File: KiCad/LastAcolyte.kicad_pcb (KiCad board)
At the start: 2 copper layers, 170 x 170 mm, 290 parts, among them J1 USB_B, J2 Mini-DIN-6, J3 AudioJack3, J4 DB15_Female_HighDensity, J5 Conn-01x06, J6 Conn_01x02, J7 Conn_02x20_Odd_Even, Q1 PN2222A, SW1 SW_SPDT, SW2 SW_Push, U1 W65C02SxP, U10 74HC273, U11 74HC166, U12 74HC166, U13 74HC10, U14 74HC00, U15 74HC02, U16 MCP130-xxxDxTO, U17 25LCxxx, U18 W65C22SxP, U19 74HC688, U2 AS6C4008-55PCN, U20 74HC08, U3 SST39SF040, U4 74HC161, U5 74HC590, U6 74HC590, U7 74HC590, U8 74HC245, U9 74HC377, X1 CXO_DIP8/14

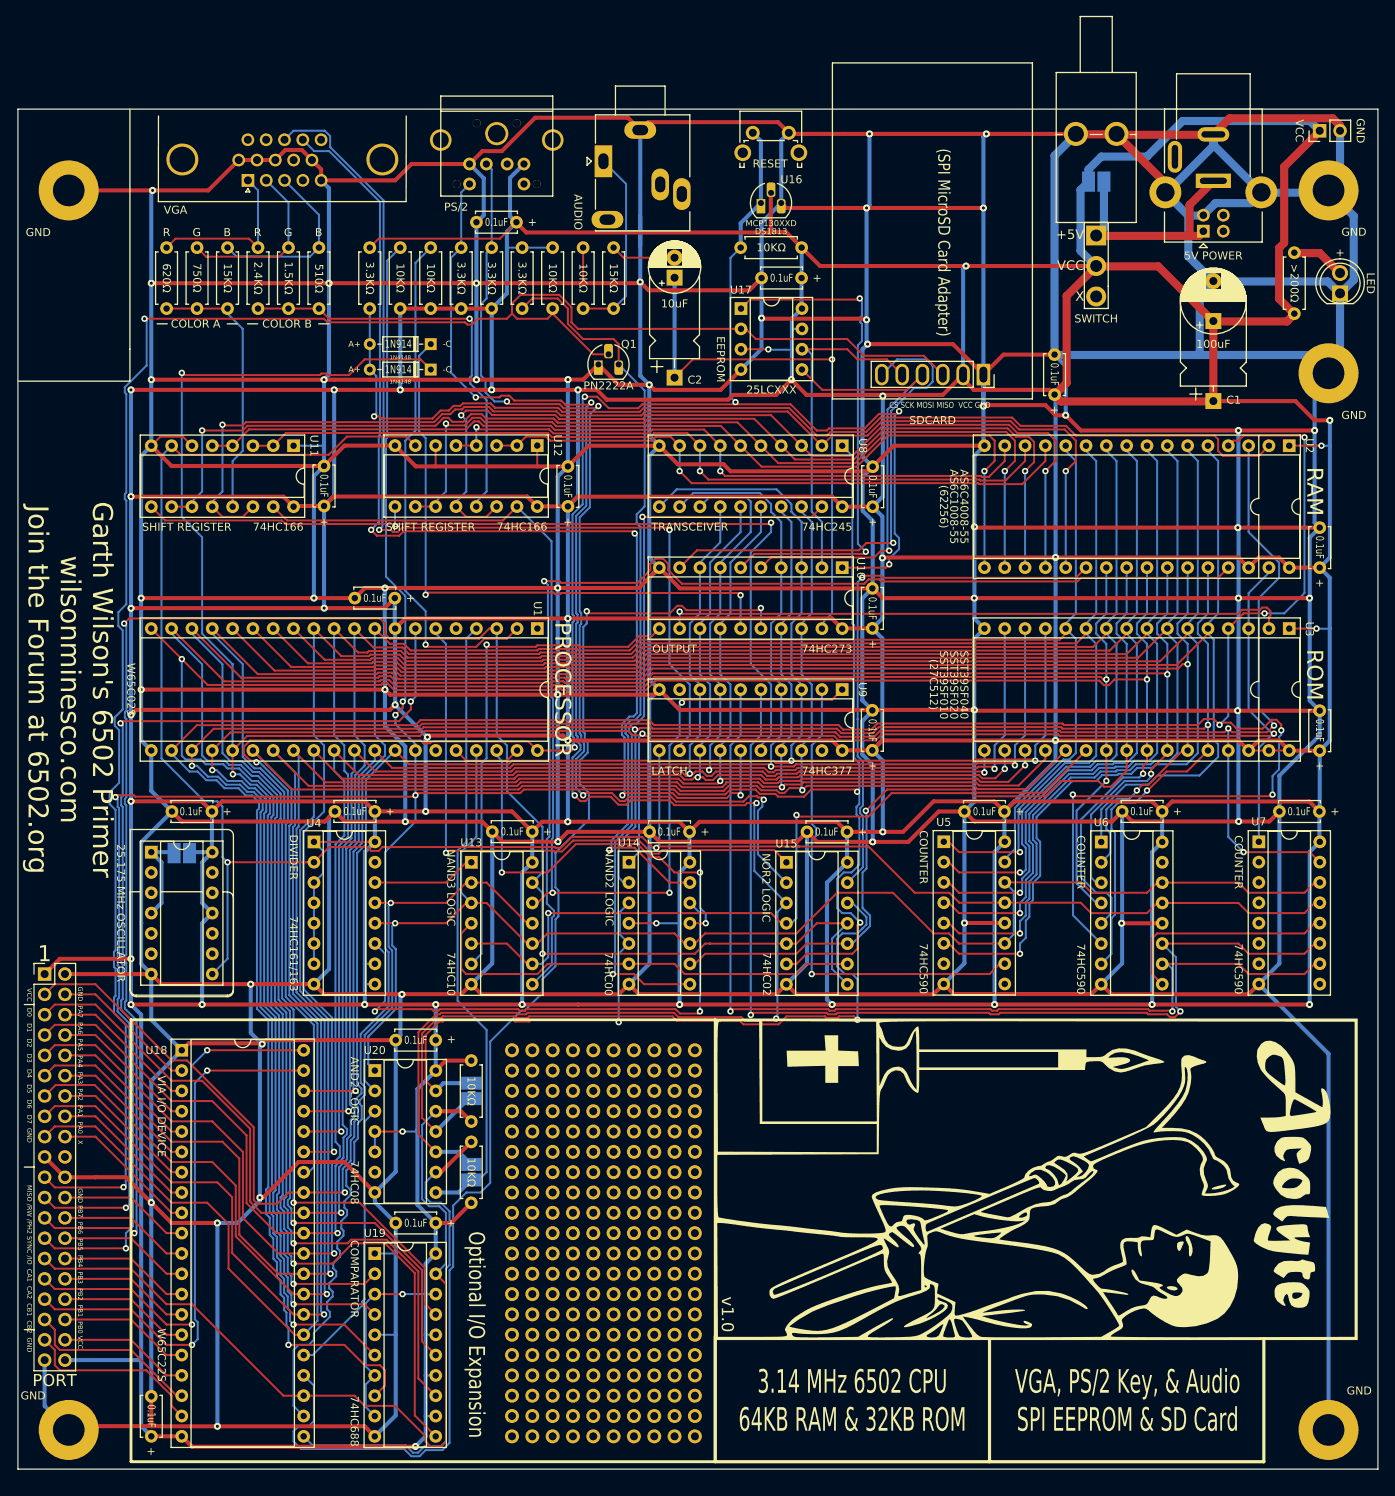
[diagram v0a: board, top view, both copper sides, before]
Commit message: Add files via upload
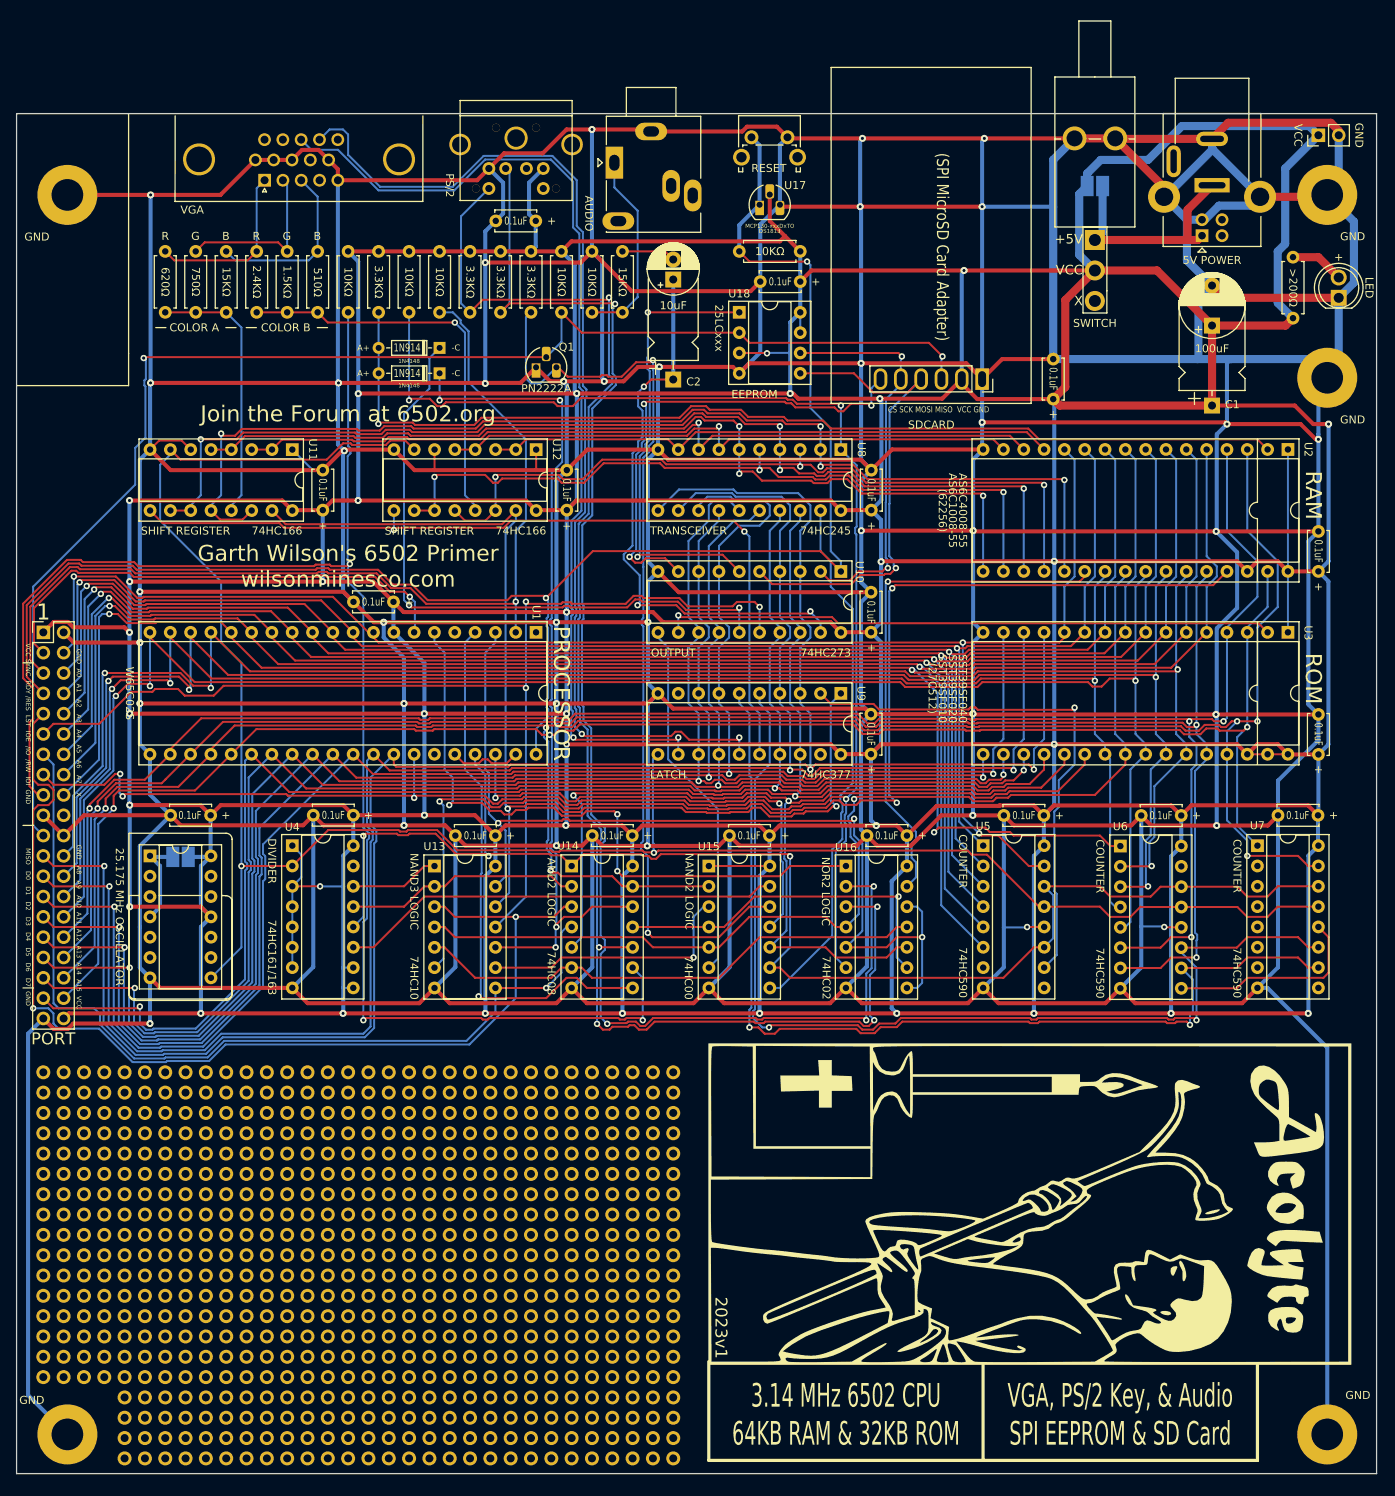
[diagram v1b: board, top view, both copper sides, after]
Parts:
- removed C23, C24: C, Capacitor_THT:C_Disc_D5.0mm_W2.5mm_P5.00mm
- removed GL: LOGO, Library:LutheranRoseLogoSmall
- removed JP3, JP4: SolderJumper_2_Open, Library:SolderJumper_Testing-2_P1.3mm_Open_Pad1.0x1.5mm
- removed R19: R_US, Resistor_THT:R_Axial_DIN0207_L6.3mm_D2.5mm_P7.62mm_Horizontal
- removed the REF** at (98.6, 160.8)
- removed the REF** at (96.0, 191.3)
- removed the REF** at (103.7, 168.4)
- removed the REF** at (101.1, 153.2)
- removed the REF** at (103.7, 191.3)
- removed the REF** at (80.8, 143.0)
- removed the REF** at (98.6, 191.3)
- removed the REF** at (98.6, 163.4)
- removed the REF** at (85.9, 163.4)
- removed the REF** at (93.5, 165.9)
- removed the REF** at (98.6, 181.1)
- removed the REF** at (83.3, 173.5)
- removed the REF** at (98.6, 176.1)
- removed the REF** at (88.4, 155.7)
- removed the REF** at (96.0, 171.0)
- removed the REF** at (88.4, 191.3)
- removed the REF** at (101.1, 188.8)
- removed the REF** at (93.5, 163.4)
- removed the REF** at (91.0, 165.9)
- removed the REF** at (83.3, 145.6)
- removed the REF** at (93.5, 155.7)
- removed the REF** at (88.4, 181.1)
- removed the REF** at (88.4, 178.6)
- removed the REF** at (80.8, 153.2)
- removed the REF** at (91.0, 183.7)
- removed the REF** at (96.0, 181.1)
- removed the REF** at (88.4, 176.1)
- removed the REF** at (103.7, 163.4)
- removed the REF** at (101.1, 143.0)
- removed the REF** at (98.6, 148.1)
- removed the REF** at (103.7, 188.8)
- removed the REF** at (83.3, 143.0)
- removed the REF** at (80.8, 165.9)
- removed the REF** at (85.9, 145.6)
- removed the REF** at (91.0, 155.7)
- removed the REF** at (91.0, 150.7)
- removed the REF** at (101.1, 191.3)
- removed the REF** at (80.8, 191.3)
- removed the REF** at (83.3, 176.1)
- removed the REF** at (93.5, 158.3)
- removed the REF** at (85.9, 150.7)
- removed the REF** at (103.7, 165.9)
- removed the REF** at (93.5, 160.8)
- removed the REF** at (93.5, 181.1)
- removed the REF** at (88.4, 163.4)
- removed the REF** at (85.9, 168.4)
- removed the REF** at (88.4, 183.7)
- removed the REF** at (85.9, 148.1)
- removed the REF** at (91.0, 143.0)
- removed the REF** at (96.0, 148.1)
- removed the REF** at (98.6, 168.4)
- removed the REF** at (83.3, 171.0)
- removed the REF** at (98.6, 186.2)
- removed the REF** at (80.8, 160.8)
- removed the REF** at (83.3, 163.4)
- removed the REF** at (98.6, 150.7)
- removed the REF** at (101.1, 183.7)
- removed the REF** at (88.4, 165.9)
- removed the REF** at (88.4, 158.3)
- removed the REF** at (98.6, 165.9)
- removed the REF** at (91.0, 145.6)
- removed the REF** at (80.8, 163.4)
- removed the REF** at (96.0, 178.6)
- removed the REF** at (101.1, 178.6)
- removed the REF** at (103.7, 150.7)
- removed the REF** at (83.3, 191.3)
- removed the REF** at (83.3, 168.4)
- removed the REF** at (93.5, 178.6)
- removed the REF** at (80.8, 178.6)
- removed the REF** at (91.0, 168.4)
- removed the REF** at (91.0, 160.8)
- removed the REF** at (88.4, 153.2)
- removed the REF** at (98.6, 173.5)
- removed the REF** at (101.1, 171.0)
- removed the REF** at (88.4, 171.0)
- removed the REF** at (88.4, 168.4)
- removed the REF** at (93.5, 143.0)
- removed the REF** at (96.0, 183.7)
- removed the REF** at (93.5, 150.7)
- removed the REF** at (101.1, 173.5)
- removed the REF** at (83.3, 188.8)
- removed the REF** at (101.1, 163.4)
- removed the REF** at (101.1, 186.2)
- removed the REF** at (101.1, 150.7)
- removed the REF** at (93.5, 171.0)
- removed the REF** at (98.6, 143.0)
- removed the REF** at (85.9, 183.7)
- removed the REF** at (85.9, 176.1)
- removed the REF** at (85.9, 191.3)
- removed the REF** at (88.4, 150.7)
- removed the REF** at (80.8, 171.0)
- removed the REF** at (88.4, 148.1)
- removed the REF** at (96.0, 176.1)
- removed the REF** at (83.3, 181.1)
- removed the REF** at (85.9, 171.0)
- removed the REF** at (98.6, 183.7)
- removed the REF** at (96.0, 168.4)
- removed the REF** at (96.0, 163.4)
- removed the REF** at (98.6, 153.2)
- removed the REF** at (80.8, 168.4)
- removed the REF** at (80.8, 158.3)
- removed the REF** at (91.0, 173.5)
- removed the REF** at (83.3, 183.7)
- removed the REF** at (93.5, 145.6)
- removed the REF** at (83.3, 150.7)
- removed the REF** at (101.1, 181.1)
- removed the REF** at (85.9, 160.8)
- removed the REF** at (88.4, 145.6)
- removed the REF** at (85.9, 186.2)
- removed the REF** at (101.1, 145.6)
- removed the REF** at (91.0, 148.1)
- removed the REF** at (96.0, 158.3)
- removed the REF** at (93.5, 183.7)
- removed the REF** at (103.7, 145.6)
- removed the REF** at (91.0, 176.1)
- removed the REF** at (93.5, 176.1)
- removed the REF** at (93.5, 186.2)
- removed the REF** at (85.9, 153.2)
- removed the REF** at (91.0, 153.2)
- removed the REF** at (85.9, 155.7)
- removed the REF** at (85.9, 165.9)
- removed the REF** at (103.7, 176.1)
- removed the REF** at (83.3, 186.2)
- removed the REF** at (103.7, 143.0)
- removed the REF** at (80.8, 173.5)
- removed the REF** at (96.0, 145.6)
- removed the REF** at (96.0, 153.2)
- removed the REF** at (103.7, 158.3)
- removed the REF** at (83.3, 158.3)
- removed the REF** at (93.5, 153.2)
- removed the REF** at (85.9, 143.0)
- removed the REF** at (91.0, 186.2)
- removed the REF** at (96.0, 155.7)
- removed the REF** at (98.6, 188.8)
- removed the REF** at (96.0, 160.8)
- removed the REF** at (83.3, 165.9)
- removed the REF** at (103.7, 153.2)
- removed the REF** at (103.7, 160.8)
- removed the REF** at (103.7, 178.6)
- removed the REF** at (91.0, 163.4)
- removed the REF** at (80.8, 176.1)
- removed the REF** at (85.9, 173.5)
- removed the REF** at (93.5, 168.4)
- removed the REF** at (91.0, 178.6)
- removed the REF** at (88.4, 143.0)
- removed the REF** at (96.0, 188.8)
- removed the REF** at (93.5, 191.3)
- removed the REF** at (96.0, 150.7)
- removed the REF** at (101.1, 158.3)
- removed the REF** at (101.1, 168.4)
- removed the REF** at (91.0, 158.3)
- removed the REF** at (103.7, 173.5)
- removed the REF** at (85.9, 188.8)
- removed the REF** at (101.1, 165.9)
- removed the REF** at (80.8, 183.7)
- removed the REF** at (80.8, 186.2)
- removed the REF** at (101.1, 160.8)
- removed the REF** at (88.4, 188.8)
- removed the REF** at (80.8, 155.7)
- removed the REF** at (83.3, 148.1)
- removed the REF** at (93.5, 173.5)
- removed the REF** at (85.9, 181.1)
- removed the REF** at (98.6, 171.0)
- removed the REF** at (83.3, 178.6)
- removed the REF** at (93.5, 148.1)
- removed the REF** at (103.7, 183.7)
- removed the REF** at (83.3, 153.2)
- removed the REF** at (93.5, 188.8)
- removed the REF** at (88.4, 173.5)
- removed the REF** at (80.8, 181.1)
- removed the REF** at (103.7, 181.1)
- removed the REF** at (80.8, 188.8)
- removed the REF** at (80.8, 148.1)
- removed the REF** at (103.7, 148.1)
- removed the REF** at (98.6, 178.6)
- removed the REF** at (80.8, 150.7)
- removed the REF** at (103.7, 155.7)
- removed the REF** at (103.7, 186.2)
- removed the REF** at (103.7, 171.0)
- removed the REF** at (91.0, 188.8)
- removed the REF** at (101.1, 148.1)
- removed the REF** at (96.0, 173.5)
- removed the REF** at (96.0, 186.2)
- removed the REF** at (101.1, 176.1)
- removed the REF** at (85.9, 178.6)
- removed the REF** at (91.0, 191.3)
- removed the REF** at (98.6, 145.6)
- removed the REF** at (88.4, 160.8)
- removed the REF** at (101.1, 155.7)
- removed the REF** at (91.0, 181.1)
- removed the REF** at (80.8, 145.6)
- removed the REF** at (83.3, 155.7)
- removed the REF** at (98.6, 155.7)
- removed the REF** at (83.3, 160.8)
- removed the REF** at (96.0, 165.9)
- removed the REF** at (98.6, 158.3)
- removed the REF** at (88.4, 186.2)
- removed the REF** at (91.0, 171.0)
- removed the REF** at (85.9, 158.3)
- removed the REF** at (96.0, 143.0)
- removed U19: 74HC688, Package_DIP:DIP-20_W7.62mm_Socket
- removed U20: 74HC08, Package_DIP:DIP-14_W7.62mm_Socket
- added G995: LOGO, Library:LutheranRosePD, B.Cu at (133.3, 40.6)
- added G997: LOGO, Library:Mystery, B.Cu at (156.8, 59.1)
- added REF**: CustomTestPoint, Library:CustomTestPoint, F.Cu at (37.5, 156.0)
- added REF**: CustomTestPoint, Library:CustomTestPoint, F.Cu at (57.8, 166.1)
- added REF**: CustomTestPoint, Library:CustomTestPoint, F.Cu at (95.9, 183.9)
- added REF**: CustomTestPoint, Library:CustomTestPoint, F.Cu at (24.8, 156.0)
- added REF**: CustomTestPoint, Library:CustomTestPoint, F.Cu at (75.6, 183.9)
- added REF**: CustomTestPoint, Library:CustomTestPoint, F.Cu at (93.3, 181.4)
- added REF**: CustomTestPoint, Library:CustomTestPoint, F.Cu at (83.2, 176.3)
- added REF**: CustomTestPoint, Library:CustomTestPoint, F.Cu at (24.8, 166.1)
- added REF**: CustomTestPoint, Library:CustomTestPoint, F.Cu at (62.9, 145.8)
- added REF**: CustomTestPoint, Library:CustomTestPoint, F.Cu at (70.5, 158.5)
- added REF**: CustomTestPoint, Library:CustomTestPoint, F.Cu at (93.3, 145.8)
- added REF**: CustomTestPoint, Library:CustomTestPoint, F.Cu at (55.2, 171.2)
- added REF**: CustomTestPoint, Library:CustomTestPoint, F.Cu at (95.9, 186.4)
- added REF**: CustomTestPoint, Library:CustomTestPoint, F.Cu at (83.2, 166.1)
- added REF**: CustomTestPoint, Library:CustomTestPoint, F.Cu at (70.5, 186.4)
- added REF**: CustomTestPoint, Library:CustomTestPoint, F.Cu at (95.9, 158.5)
- added REF**: CustomTestPoint, Library:CustomTestPoint, F.Cu at (47.6, 186.4)
- added REF**: CustomTestPoint, Library:CustomTestPoint, F.Cu at (32.4, 150.9)
- added REF**: CustomTestPoint, Library:CustomTestPoint, F.Cu at (85.7, 181.4)
- added REF**: CustomTestPoint, Library:CustomTestPoint, F.Cu at (55.2, 181.4)
- added REF**: CustomTestPoint, Library:CustomTestPoint, F.Cu at (88.3, 156.0)
- added REF**: CustomTestPoint, Library:CustomTestPoint, F.Cu at (27.3, 181.4)
- added REF**: CustomTestPoint, Library:CustomTestPoint, F.Cu at (29.8, 148.3)
- added REF**: CustomTestPoint, Library:CustomTestPoint, F.Cu at (57.8, 161.0)
- added REF**: CustomTestPoint, Library:CustomTestPoint, F.Cu at (78.1, 163.6)
- added REF**: CustomTestPoint, Library:CustomTestPoint, F.Cu at (88.3, 186.4)
- added REF**: CustomTestPoint, Library:CustomTestPoint, F.Cu at (37.5, 168.7)
- added REF**: CustomTestPoint, Library:CustomTestPoint, F.Cu at (34.9, 191.5)
- added REF**: CustomTestPoint, Library:CustomTestPoint, F.Cu at (47.6, 153.4)
- added REF**: CustomTestPoint, Library:CustomTestPoint, F.Cu at (50.2, 181.4)
- added REF**: CustomTestPoint, Library:CustomTestPoint, F.Cu at (83.2, 186.4)
- added REF**: CustomTestPoint, Library:CustomTestPoint, F.Cu at (67.9, 163.6)
- added REF**: CustomTestPoint, Library:CustomTestPoint, F.Cu at (73.0, 191.5)
- added REF**: CustomTestPoint, Library:CustomTestPoint, F.Cu at (40.0, 171.2)
- added REF**: CustomTestPoint, Library:CustomTestPoint, F.Cu at (34.9, 166.1)
- added REF**: CustomTestPoint, Library:CustomTestPoint, F.Cu at (98.4, 176.3)
- added REF**: CustomTestPoint, Library:CustomTestPoint, F.Cu at (40.0, 168.7)
- added REF**: CustomTestPoint, Library:CustomTestPoint, F.Cu at (27.3, 166.1)
- added REF**: CustomTestPoint, Library:CustomTestPoint, F.Cu at (67.9, 161.0)
- added REF**: CustomTestPoint, Library:CustomTestPoint, F.Cu at (78.1, 166.1)
- added REF**: CustomTestPoint, Library:CustomTestPoint, F.Cu at (93.3, 183.9)
- added REF**: CustomTestPoint, Library:CustomTestPoint, F.Cu at (65.4, 148.3)
- added REF**: CustomTestPoint, Library:CustomTestPoint, F.Cu at (55.2, 148.3)
- added REF**: CustomTestPoint, Library:CustomTestPoint, F.Cu at (50.2, 168.7)
- added REF**: CustomTestPoint, Library:CustomTestPoint, F.Cu at (67.9, 191.5)
- added REF**: CustomTestPoint, Library:CustomTestPoint, F.Cu at (85.7, 194.1)
- added REF**: CustomTestPoint, Library:CustomTestPoint, F.Cu at (52.7, 166.1)
- added REF**: CustomTestPoint, Library:CustomTestPoint, F.Cu at (27.3, 171.2)
- added REF**: CustomTestPoint, Library:CustomTestPoint, F.Cu at (50.2, 173.7)
- added REF**: CustomTestPoint, Library:CustomTestPoint, F.Cu at (98.4, 150.9)
- added REF**: CustomTestPoint, Library:CustomTestPoint, F.Cu at (45.1, 194.1)
- added REF**: CustomTestPoint, Library:CustomTestPoint, F.Cu at (22.2, 156.0)
- added REF**: CustomTestPoint, Library:CustomTestPoint, F.Cu at (42.5, 176.3)
- added REF**: CustomTestPoint, Library:CustomTestPoint, F.Cu at (40.0, 194.1)
- added REF**: CustomTestPoint, Library:CustomTestPoint, F.Cu at (85.7, 158.5)
- added REF**: CustomTestPoint, Library:CustomTestPoint, F.Cu at (29.8, 163.6)
- added REF**: CustomTestPoint, Library:CustomTestPoint, F.Cu at (93.3, 173.7)
- added REF**: CustomTestPoint, Library:CustomTestPoint, F.Cu at (32.4, 163.6)
- added REF**: CustomTestPoint, Library:CustomTestPoint, F.Cu at (60.3, 168.7)
- added REF**: CustomTestPoint, Library:CustomTestPoint, F.Cu at (34.9, 168.7)
- added REF**: CustomTestPoint, Library:CustomTestPoint, F.Cu at (101.0, 191.5)
- added REF**: CustomTestPoint, Library:CustomTestPoint, F.Cu at (83.2, 194.1)
- added REF**: CustomTestPoint, Library:CustomTestPoint, F.Cu at (75.6, 181.4)
- added REF**: CustomTestPoint, Library:CustomTestPoint, F.Cu at (45.1, 189.0)
- added REF**: CustomTestPoint, Library:CustomTestPoint, F.Cu at (90.8, 176.3)
- added REF**: CustomTestPoint, Library:CustomTestPoint, F.Cu at (78.1, 173.7)
- added REF**: CustomTestPoint, Library:CustomTestPoint, F.Cu at (32.4, 178.8)
- added REF**: CustomTestPoint, Library:CustomTestPoint, F.Cu at (90.8, 153.4)
- added REF**: CustomTestPoint, Library:CustomTestPoint, F.Cu at (67.9, 148.3)
- added REF**: CustomTestPoint, Library:CustomTestPoint, F.Cu at (37.5, 171.2)
- added REF**: CustomTestPoint, Library:CustomTestPoint, F.Cu at (98.4, 171.2)
- added REF**: CustomTestPoint, Library:CustomTestPoint, F.Cu at (60.3, 158.5)
- added REF**: CustomTestPoint, Library:CustomTestPoint, F.Cu at (65.4, 191.5)
- added REF**: CustomTestPoint, Library:CustomTestPoint, F.Cu at (67.9, 178.8)
- added REF**: CustomTestPoint, Library:CustomTestPoint, F.Cu at (75.6, 166.1)
- added REF**: CustomTestPoint, Library:CustomTestPoint, F.Cu at (101.0, 194.1)
- added REF**: CustomTestPoint, Library:CustomTestPoint, F.Cu at (88.3, 171.2)
- added REF**: CustomTestPoint, Library:CustomTestPoint, F.Cu at (34.9, 176.3)
- added REF**: CustomTestPoint, Library:CustomTestPoint, F.Cu at (88.3, 153.4)
- added REF**: CustomTestPoint, Library:CustomTestPoint, F.Cu at (90.8, 181.4)
- added REF**: CustomTestPoint, Library:CustomTestPoint, F.Cu at (37.5, 166.1)
- added REF**: CustomTestPoint, Library:CustomTestPoint, F.Cu at (80.6, 168.7)
- added REF**: CustomTestPoint, Library:CustomTestPoint, F.Cu at (78.1, 171.2)
- added REF**: CustomTestPoint, Library:CustomTestPoint, F.Cu at (95.9, 173.7)
- added REF**: CustomTestPoint, Library:CustomTestPoint, F.Cu at (52.7, 189.0)
- added REF**: CustomTestPoint, Library:CustomTestPoint, F.Cu at (83.2, 163.6)
- added REF**: CustomTestPoint, Library:CustomTestPoint, F.Cu at (42.5, 153.4)
- added REF**: CustomTestPoint, Library:CustomTestPoint, F.Cu at (90.8, 145.8)
- added REF**: CustomTestPoint, Library:CustomTestPoint, F.Cu at (57.8, 153.4)
- added REF**: CustomTestPoint, Library:CustomTestPoint, F.Cu at (55.2, 191.5)
- added REF**: CustomTestPoint, Library:CustomTestPoint, F.Cu at (34.9, 156.0)
- added REF**: CustomTestPoint, Library:CustomTestPoint, F.Cu at (67.9, 194.1)
- added REF**: CustomTestPoint, Library:CustomTestPoint, F.Cu at (88.3, 148.3)
- added REF**: CustomTestPoint, Library:CustomTestPoint, F.Cu at (73.0, 145.8)
- added REF**: CustomTestPoint, Library:CustomTestPoint, F.Cu at (24.8, 176.3)
- added REF**: CustomTestPoint, Library:CustomTestPoint, F.Cu at (70.5, 153.4)
- added REF**: CustomTestPoint, Library:CustomTestPoint, F.Cu at (45.1, 183.9)
- added REF**: CustomTestPoint, Library:CustomTestPoint, F.Cu at (80.6, 158.5)
- added REF**: CustomTestPoint, Library:CustomTestPoint, F.Cu at (67.9, 145.8)
- added REF**: CustomTestPoint, Library:CustomTestPoint, F.Cu at (67.9, 158.5)
- added REF**: CustomTestPoint, Library:CustomTestPoint, F.Cu at (45.1, 171.2)
- added REF**: CustomTestPoint, Library:CustomTestPoint, F.Cu at (78.1, 148.3)
- added REF**: CustomTestPoint, Library:CustomTestPoint, F.Cu at (42.5, 161.0)
- added REF**: CustomTestPoint, Library:CustomTestPoint, F.Cu at (65.4, 168.7)
- added REF**: CustomTestPoint, Library:CustomTestPoint, F.Cu at (73.0, 173.7)
- added REF**: CustomTestPoint, Library:CustomTestPoint, F.Cu at (75.6, 168.7)
- added REF**: CustomTestPoint, Library:CustomTestPoint, F.Cu at (73.0, 176.3)
- added REF**: CustomTestPoint, Library:CustomTestPoint, F.Cu at (24.8, 158.5)
- added REF**: CustomTestPoint, Library:CustomTestPoint, F.Cu at (22.2, 176.3)
- added REF**: CustomTestPoint, Library:CustomTestPoint, F.Cu at (65.4, 176.3)
- added REF**: CustomTestPoint, Library:CustomTestPoint, F.Cu at (88.3, 145.8)
- added REF**: CustomTestPoint, Library:CustomTestPoint, F.Cu at (98.4, 156.0)
- added REF**: CustomTestPoint, Library:CustomTestPoint, F.Cu at (80.6, 173.7)
- added REF**: CustomTestPoint, Library:CustomTestPoint, F.Cu at (73.0, 148.3)
- added REF**: CustomTestPoint, Library:CustomTestPoint, F.Cu at (60.3, 183.9)
- added REF**: CustomTestPoint, Library:CustomTestPoint, F.Cu at (45.1, 186.4)
- added REF**: CustomTestPoint, Library:CustomTestPoint, F.Cu at (34.9, 181.4)
- added REF**: CustomTestPoint, Library:CustomTestPoint, F.Cu at (24.8, 161.0)
- added REF**: CustomTestPoint, Library:CustomTestPoint, F.Cu at (101.0, 183.9)
- added REF**: CustomTestPoint, Library:CustomTestPoint, F.Cu at (50.2, 186.4)
- added REF**: CustomTestPoint, Library:CustomTestPoint, F.Cu at (70.5, 168.7)
- added REF**: CustomTestPoint, Library:CustomTestPoint, F.Cu at (80.6, 161.0)
- added REF**: CustomTestPoint, Library:CustomTestPoint, F.Cu at (55.2, 161.0)
- added REF**: CustomTestPoint, Library:CustomTestPoint, F.Cu at (32.4, 158.5)
- added REF**: CustomTestPoint, Library:CustomTestPoint, F.Cu at (85.7, 171.2)
- added REF**: CustomTestPoint, Library:CustomTestPoint, F.Cu at (37.5, 145.8)
- added REF**: CustomTestPoint, Library:CustomTestPoint, F.Cu at (65.4, 183.9)
- added REF**: CustomTestPoint, Library:CustomTestPoint, F.Cu at (65.4, 173.7)
- added REF**: CustomTestPoint, Library:CustomTestPoint, F.Cu at (67.9, 171.2)
- added REF**: CustomTestPoint, Library:CustomTestPoint, F.Cu at (32.4, 189.0)
- added REF**: CustomTestPoint, Library:CustomTestPoint, F.Cu at (22.2, 145.8)
- added REF**: CustomTestPoint, Library:CustomTestPoint, F.Cu at (93.3, 166.1)
- added REF**: CustomTestPoint, Library:CustomTestPoint, F.Cu at (98.4, 181.4)
- added REF**: CustomTestPoint, Library:CustomTestPoint, F.Cu at (70.5, 191.5)
- added REF**: CustomTestPoint, Library:CustomTestPoint, F.Cu at (34.9, 173.7)
- added REF**: CustomTestPoint, Library:CustomTestPoint, F.Cu at (67.9, 153.4)
- added REF**: CustomTestPoint, Library:CustomTestPoint, F.Cu at (62.9, 171.2)
- added REF**: CustomTestPoint, Library:CustomTestPoint, F.Cu at (101.0, 156.0)
- added REF**: CustomTestPoint, Library:CustomTestPoint, F.Cu at (70.5, 148.3)
- added REF**: CustomTestPoint, Library:CustomTestPoint, F.Cu at (88.3, 181.4)
- added REF**: CustomTestPoint, Library:CustomTestPoint, F.Cu at (47.6, 178.8)
- added REF**: CustomTestPoint, Library:CustomTestPoint, F.Cu at (57.8, 173.7)
- added REF**: CustomTestPoint, Library:CustomTestPoint, F.Cu at (47.6, 168.7)
- added REF**: CustomTestPoint, Library:CustomTestPoint, F.Cu at (27.3, 150.9)
- added REF**: CustomTestPoint, Library:CustomTestPoint, F.Cu at (27.3, 173.7)
- added REF**: CustomTestPoint, Library:CustomTestPoint, F.Cu at (75.6, 148.3)
- added REF**: CustomTestPoint, Library:CustomTestPoint, F.Cu at (88.3, 176.3)
- added REF**: CustomTestPoint, Library:CustomTestPoint, F.Cu at (42.5, 158.5)
- added REF**: CustomTestPoint, Library:CustomTestPoint, F.Cu at (90.8, 148.3)
- added REF**: CustomTestPoint, Library:CustomTestPoint, F.Cu at (34.9, 183.9)
- added REF**: CustomTestPoint, Library:CustomTestPoint, F.Cu at (83.2, 161.0)
- added REF**: CustomTestPoint, Library:CustomTestPoint, F.Cu at (50.2, 148.3)
- added REF**: CustomTestPoint, Library:CustomTestPoint, F.Cu at (90.8, 161.0)
- added REF**: CustomTestPoint, Library:CustomTestPoint, F.Cu at (101.0, 158.5)
- added REF**: CustomTestPoint, Library:CustomTestPoint, F.Cu at (98.4, 166.1)
- added REF**: CustomTestPoint, Library:CustomTestPoint, F.Cu at (62.9, 176.3)
- added REF**: CustomTestPoint, Library:CustomTestPoint, F.Cu at (37.5, 178.8)
- added REF**: CustomTestPoint, Library:CustomTestPoint, F.Cu at (88.3, 191.5)
- added REF**: CustomTestPoint, Library:CustomTestPoint, F.Cu at (98.4, 189.0)
- added REF**: CustomTestPoint, Library:CustomTestPoint, F.Cu at (40.0, 178.8)
- added REF**: CustomTestPoint, Library:CustomTestPoint, F.Cu at (80.6, 183.9)
- added REF**: CustomTestPoint, Library:CustomTestPoint, F.Cu at (24.8, 183.9)
- added REF**: CustomTestPoint, Library:CustomTestPoint, F.Cu at (80.6, 181.4)
- added REF**: CustomTestPoint, Library:CustomTestPoint, F.Cu at (52.7, 191.5)
- added REF**: CustomTestPoint, Library:CustomTestPoint, F.Cu at (50.2, 183.9)
- added REF**: CustomTestPoint, Library:CustomTestPoint, F.Cu at (22.2, 158.5)
- added REF**: CustomTestPoint, Library:CustomTestPoint, F.Cu at (55.2, 150.9)
- added REF**: CustomTestPoint, Library:CustomTestPoint, F.Cu at (101.0, 161.0)
- added REF**: CustomTestPoint, Library:CustomTestPoint, F.Cu at (47.6, 194.1)
- added REF**: CustomTestPoint, Library:CustomTestPoint, F.Cu at (40.0, 173.7)
- added REF**: CustomTestPoint, Library:CustomTestPoint, F.Cu at (37.5, 161.0)
- added REF**: CustomTestPoint, Library:CustomTestPoint, F.Cu at (88.3, 161.0)
- added REF**: CustomTestPoint, Library:CustomTestPoint, F.Cu at (65.4, 150.9)
- added REF**: CustomTestPoint, Library:CustomTestPoint, F.Cu at (47.6, 148.3)
- added REF**: CustomTestPoint, Library:CustomTestPoint, F.Cu at (52.7, 168.7)
- added REF**: CustomTestPoint, Library:CustomTestPoint, F.Cu at (42.5, 163.6)
- added REF**: CustomTestPoint, Library:CustomTestPoint, F.Cu at (88.3, 189.0)
- added REF**: CustomTestPoint, Library:CustomTestPoint, F.Cu at (37.5, 153.4)
- added REF**: CustomTestPoint, Library:CustomTestPoint, F.Cu at (45.1, 161.0)
- added REF**: CustomTestPoint, Library:CustomTestPoint, F.Cu at (75.6, 163.6)
- added REF**: CustomTestPoint, Library:CustomTestPoint, F.Cu at (42.5, 183.9)
- added REF**: CustomTestPoint, Library:CustomTestPoint, F.Cu at (65.4, 186.4)
- added REF**: CustomTestPoint, Library:CustomTestPoint, F.Cu at (93.3, 156.0)
- added REF**: CustomTestPoint, Library:CustomTestPoint, F.Cu at (22.2, 150.9)
- added REF**: CustomTestPoint, Library:CustomTestPoint, F.Cu at (83.2, 183.9)
- added REF**: CustomTestPoint, Library:CustomTestPoint, F.Cu at (57.8, 189.0)
- added REF**: CustomTestPoint, Library:CustomTestPoint, F.Cu at (93.3, 158.5)
- added REF**: CustomTestPoint, Library:CustomTestPoint, F.Cu at (22.2, 166.1)
- added REF**: CustomTestPoint, Library:CustomTestPoint, F.Cu at (85.7, 189.0)
- added REF**: CustomTestPoint, Library:CustomTestPoint, F.Cu at (80.6, 178.8)
- added REF**: CustomTestPoint, Library:CustomTestPoint, F.Cu at (47.6, 173.7)
- added REF**: CustomTestPoint, Library:CustomTestPoint, F.Cu at (101.0, 181.4)
- added REF**: CustomTestPoint, Library:CustomTestPoint, F.Cu at (55.2, 176.3)
- added REF**: CustomTestPoint, Library:CustomTestPoint, F.Cu at (95.9, 148.3)
- added REF**: CustomTestPoint, Library:CustomTestPoint, F.Cu at (34.9, 161.0)
- added REF**: CustomTestPoint, Library:CustomTestPoint, F.Cu at (45.1, 153.4)
- added REF**: CustomTestPoint, Library:CustomTestPoint, F.Cu at (62.9, 173.7)
- added REF**: CustomTestPoint, Library:CustomTestPoint, F.Cu at (93.3, 150.9)
- added REF**: CustomTestPoint, Library:CustomTestPoint, F.Cu at (57.8, 163.6)
- added REF**: CustomTestPoint, Library:CustomTestPoint, F.Cu at (34.9, 145.8)
- added REF**: CustomTestPoint, Library:CustomTestPoint, F.Cu at (37.5, 194.1)
- added REF**: CustomTestPoint, Library:CustomTestPoint, F.Cu at (80.6, 148.3)
- added REF**: CustomTestPoint, Library:CustomTestPoint, F.Cu at (90.8, 189.0)
- added REF**: CustomTestPoint, Library:CustomTestPoint, F.Cu at (57.8, 183.9)
- added REF**: CustomTestPoint, Library:CustomTestPoint, F.Cu at (73.0, 171.2)
- added REF**: CustomTestPoint, Library:CustomTestPoint, F.Cu at (90.8, 168.7)
- added REF**: CustomTestPoint, Library:CustomTestPoint, F.Cu at (95.9, 156.0)
- added REF**: CustomTestPoint, Library:CustomTestPoint, F.Cu at (98.4, 173.7)
- added REF**: CustomTestPoint, Library:CustomTestPoint, F.Cu at (37.5, 173.7)
- added REF**: CustomTestPoint, Library:CustomTestPoint, F.Cu at (52.7, 171.2)
- added REF**: CustomTestPoint, Library:CustomTestPoint, F.Cu at (65.4, 194.1)
- added REF**: CustomTestPoint, Library:CustomTestPoint, F.Cu at (70.5, 166.1)
- added REF**: CustomTestPoint, Library:CustomTestPoint, F.Cu at (60.3, 189.0)
- added REF**: CustomTestPoint, Library:CustomTestPoint, F.Cu at (95.9, 181.4)
- added REF**: CustomTestPoint, Library:CustomTestPoint, F.Cu at (40.0, 189.0)
- added REF**: CustomTestPoint, Library:CustomTestPoint, F.Cu at (95.9, 163.6)
- added REF**: CustomTestPoint, Library:CustomTestPoint, F.Cu at (47.6, 163.6)
- added REF**: CustomTestPoint, Library:CustomTestPoint, F.Cu at (52.7, 194.1)
- added REF**: CustomTestPoint, Library:CustomTestPoint, F.Cu at (52.7, 145.8)
- added REF**: CustomTestPoint, Library:CustomTestPoint, F.Cu at (24.8, 173.7)
- added REF**: CustomTestPoint, Library:CustomTestPoint, F.Cu at (75.6, 153.4)
- added REF**: CustomTestPoint, Library:CustomTestPoint, F.Cu at (90.8, 150.9)
- added REF**: CustomTestPoint, Library:CustomTestPoint, F.Cu at (52.7, 153.4)
- added REF**: CustomTestPoint, Library:CustomTestPoint, F.Cu at (78.1, 183.9)
- added REF**: CustomTestPoint, Library:CustomTestPoint, F.Cu at (42.5, 166.1)
- added REF**: CustomTestPoint, Library:CustomTestPoint, F.Cu at (70.5, 173.7)
- added REF**: CustomTestPoint, Library:CustomTestPoint, F.Cu at (57.8, 186.4)
- added REF**: CustomTestPoint, Library:CustomTestPoint, F.Cu at (62.9, 153.4)
- added REF**: CustomTestPoint, Library:CustomTestPoint, F.Cu at (47.6, 183.9)
- added REF**: CustomTestPoint, Library:CustomTestPoint, F.Cu at (37.5, 181.4)
- added REF**: CustomTestPoint, Library:CustomTestPoint, F.Cu at (65.4, 153.4)
- added REF**: CustomTestPoint, Library:CustomTestPoint, F.Cu at (32.4, 191.5)
- added REF**: CustomTestPoint, Library:CustomTestPoint, F.Cu at (75.6, 145.8)
- added REF**: CustomTestPoint, Library:CustomTestPoint, F.Cu at (24.8, 178.8)
- added REF**: CustomTestPoint, Library:CustomTestPoint, F.Cu at (47.6, 158.5)
- added REF**: CustomTestPoint, Library:CustomTestPoint, F.Cu at (95.9, 161.0)
- added REF**: CustomTestPoint, Library:CustomTestPoint, F.Cu at (57.8, 158.5)
- added REF**: CustomTestPoint, Library:CustomTestPoint, F.Cu at (95.9, 171.2)
- added REF**: CustomTestPoint, Library:CustomTestPoint, F.Cu at (70.5, 163.6)
- added REF**: CustomTestPoint, Library:CustomTestPoint, F.Cu at (98.4, 153.4)
- added REF**: CustomTestPoint, Library:CustomTestPoint, F.Cu at (93.3, 189.0)
- added REF**: CustomTestPoint, Library:CustomTestPoint, F.Cu at (85.7, 156.0)
- added REF**: CustomTestPoint, Library:CustomTestPoint, F.Cu at (29.8, 150.9)
- added REF**: CustomTestPoint, Library:CustomTestPoint, F.Cu at (73.0, 194.1)
- added REF**: CustomTestPoint, Library:CustomTestPoint, F.Cu at (75.6, 171.2)
- added REF**: CustomTestPoint, Library:CustomTestPoint, F.Cu at (101.0, 173.7)
- added REF**: CustomTestPoint, Library:CustomTestPoint, F.Cu at (60.3, 156.0)
- added REF**: CustomTestPoint, Library:CustomTestPoint, F.Cu at (83.2, 171.2)
- added REF**: CustomTestPoint, Library:CustomTestPoint, F.Cu at (90.8, 186.4)
- added REF**: CustomTestPoint, Library:CustomTestPoint, F.Cu at (27.3, 176.3)
- added REF**: CustomTestPoint, Library:CustomTestPoint, F.Cu at (62.9, 150.9)
- added REF**: CustomTestPoint, Library:CustomTestPoint, F.Cu at (62.9, 191.5)
- added REF**: CustomTestPoint, Library:CustomTestPoint, F.Cu at (101.0, 150.9)
- added REF**: CustomTestPoint, Library:CustomTestPoint, F.Cu at (52.7, 181.4)
- added REF**: CustomTestPoint, Library:CustomTestPoint, F.Cu at (50.2, 171.2)
- added REF**: CustomTestPoint, Library:CustomTestPoint, F.Cu at (55.2, 153.4)
- added REF**: CustomTestPoint, Library:CustomTestPoint, F.Cu at (60.3, 178.8)
- added REF**: CustomTestPoint, Library:CustomTestPoint, F.Cu at (52.7, 176.3)
- added REF**: CustomTestPoint, Library:CustomTestPoint, F.Cu at (37.5, 158.5)
- added REF**: CustomTestPoint, Library:CustomTestPoint, F.Cu at (40.0, 163.6)
- added REF**: CustomTestPoint, Library:CustomTestPoint, F.Cu at (57.8, 191.5)
- added REF**: CustomTestPoint, Library:CustomTestPoint, F.Cu at (83.2, 178.8)
- added REF**: CustomTestPoint, Library:CustomTestPoint, F.Cu at (57.8, 178.8)
- added REF**: CustomTestPoint, Library:CustomTestPoint, F.Cu at (93.3, 163.6)
- added REF**: CustomTestPoint, Library:CustomTestPoint, F.Cu at (50.2, 176.3)
- added REF**: CustomTestPoint, Library:CustomTestPoint, F.Cu at (42.5, 150.9)
- added REF**: CustomTestPoint, Library:CustomTestPoint, F.Cu at (78.1, 145.8)
- added REF**: CustomTestPoint, Library:CustomTestPoint, F.Cu at (45.1, 191.5)
- added REF**: CustomTestPoint, Library:CustomTestPoint, F.Cu at (27.3, 156.0)
- added REF**: CustomTestPoint, Library:CustomTestPoint, F.Cu at (95.9, 153.4)
- added REF**: CustomTestPoint, Library:CustomTestPoint, F.Cu at (65.4, 189.0)
- added REF**: CustomTestPoint, Library:CustomTestPoint, F.Cu at (90.8, 166.1)
- added REF**: CustomTestPoint, Library:CustomTestPoint, F.Cu at (80.6, 186.4)
- added REF**: CustomTestPoint, Library:CustomTestPoint, F.Cu at (60.3, 171.2)
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- renumbered U14 to U15, U15 to U16
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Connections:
- net BANK-A renamed BANK-ROM
- net BANK-B renamed BANK-RAM
- D2 pad 2: RBK -> RAMEXP
- D3 pad 2: RBK -> RAMEXP
- J7 pad 10: PA3 -> A3
- J7 pad 11: D4 -> IO-ENABLE
- J7 pad 12: PA4 -> A4
- J7 pad 13: D5 -> ~{IO}
- J7 pad 14: PA5 -> A5
- J7 pad 15: D6 -> ~{RW}
- J7 pad 16: PA6 -> A6
- J7 pad 17: D7 -> IO-INT
- J7 pad 18: PA7 -> A7
- J7 pad 23: ~{RW} -> D0
- J7 pad 24: PB0 -> A8
- J7 pad 25: ~{PHI2} -> D1
- J7 pad 26: PB1 -> A9
- J7 pad 27: SYNC -> D2
- J7 pad 28: PB2 -> A10
- J7 pad 29: ~{IO} -> D3
- J7 pad 3: D0 -> SYNC
- J7 pad 30: PB3 -> A11
- J7 pad 31: CA1 -> D4
- J7 pad 32: PB4 -> A12
- J7 pad 33: CA2 -> D5
- J7 pad 34: PB5 -> A13
- J7 pad 35: CB1 -> D6
- J7 pad 36: PB6 -> A14
- J7 pad 37: CB2 -> D7
- J7 pad 38: PB7 -> A15
- J7 pad 4: PA0 -> A0
- J7 pad 5: D1 -> RDY
- J7 pad 6: PA1 -> A1
- J7 pad 7: D2 -> ~{RES}
- J7 pad 8: PA2 -> A2
- J7 pad 9: D3 -> LAST
- R15 pad 2: RBK -> IO-INT
- R16 pad 2: ~{RES} -> RAMEXP
- R18 pad 2: VIA-INT -> ~{RES}
- U1 pad 13: /A4 -> A4
- U1 pad 14: /A5 -> A5
- U1 pad 15: /A6 -> A6
- U1 pad 16: /A7 -> A7
- U10 pad 16: VIA-ENABLE -> IO-ENABLE
- U13 pad 10: PHI2 -> A15
- U13 pad 11: QUARTER -> IO-ENABLE
- U13 pad 3: PHI2 -> LAST
- U13 pad 4: HIGH -> ~{OE}
- U13 pad 5: ~{OE} -> RAMADDR
- U13 pad 6: ~{OUTPUT} -> ~{WE}
- U13 pad 8: ~{WE} -> ~{IO}
- U13 pad 9: ~{OE} -> ~{A14}
- U14 pad 1: ~{RES} -> PHI2
- U14 pad 2: +5V -> QUARTER
- U14 pad 3: GND -> LAST
- U15 pad 1: A15 -> +5V
- U15 pad 10: PHI2 -> ~{ROM}
- U15 pad 12: SIXTEENTH -> ~{SPI-MISO}
- U15 pad 13: ~{SPI-MISO} -> SIXTEENTH
- U15 pad 3: ~{HIGH} -> ~{A14}
- U15 pad 4: +5V -> HIGH
- U15 pad 5: ~{HIGH} -> ~{OE}
- U15 pad 6: HIGH -> ~{OUTPUT}
- U15 pad 9: ~{ROM} -> PHI2
- U16 pad 11: ~{PHI2} -> RAMADDR
- U16 pad 12: RCE -> ~{PHI2}
- U17 pad 1: SPI-EEPROM -> ~{RES}
- U17 pad 2: SPI-MISO -> +5V
- U17 pad 3: +5V -> GND
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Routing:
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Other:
- board text added: "$8000-$BFFF=RAM or I/O $C000-$FFFF=Banked ROM"
- board text added: "2023v1"
- board text added: "AUDN GND VCC VCC VCC VCC VCC VCC VCC VCC"
- board text added: "AUDT AUDT MISO /MISO KDAT KCLK RDY /RW RAME IOI"
- board text added: "BRAM"
- board text added: "Bit4=ROM-BANK Bit5=RAM-BANK Bit6=IO-ENABLE Bit7=AUDIO-OUT"
- board text added: "DIP-8 DIP-40 DIP-32 DIP-32 DIP-16 DIP-16 DIP-20 DIP-20 DIP-20 DIP-16 DIP-14 DIP-14 DIP-14 DIP-14 TO-92 DIP-8 TO-92 5mm Rad 15mm Ax 5mm Dsc 2.2V DO-35 1/4W 5% 1/4W 5% 1/4W 5% 1/4W 5% 1/4W 5% 1/4W 5% 1/4W 5% 1/4W 5% 1/4W 5% 61729 5749266-1 SJ1-3513 DSub 15 SPI Mod T1B4M7QES PTS645 2.54mm"
- board text added: "GND A0 A1 A2 A3 A4 A5 A6 A7 X"
- board text added: "GND A8 A9 A10 A11 A12 A13 A14 A15 VCC"
- board text added: "GND D7 D6 D5 D4 D3 D2 D1 D0 MISO"
- board text added: "GND IOI /RW /IO IOE LST /RES RDY SYNC VCC"
- board text added: "Garth Wilson's 6502 Primer wilsonminesco.com"
- board text added: "HALF QRT LST /OE RAD /WE GND"
- board text added: "IO must be enabled in software before use, but removes RAM from $8000-$BFFF. Interrupts from IO could interfere with PS/2 Keyboard. ENABLE jumper used by Oscillator. BYPASS jumper used in absense of Switch. USB-to-PS/2 adapters will not work. VGA-to-HDMI adapters should work."
- board text added: "Input is through 6502 interrupts: /IRQ = KEY-CLK AND IO-INT /NMI = KEY-CLK NOR KEY-DATA /SO = SPI-MISO (CLV, NOP, then BVS)"
- board text added: "Intended I/O expansion: W65C22S DIP-40."
- board text added: "Join the Forum at 6502.org"
- board text added: "MISO D0 D1 D2 D3 D4 D5 D6 D7 GND"
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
